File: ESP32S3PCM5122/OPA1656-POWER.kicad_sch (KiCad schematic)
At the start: 29 parts, among them IC6 TPS65133, U1 TPS7A39, U3 OPA1656

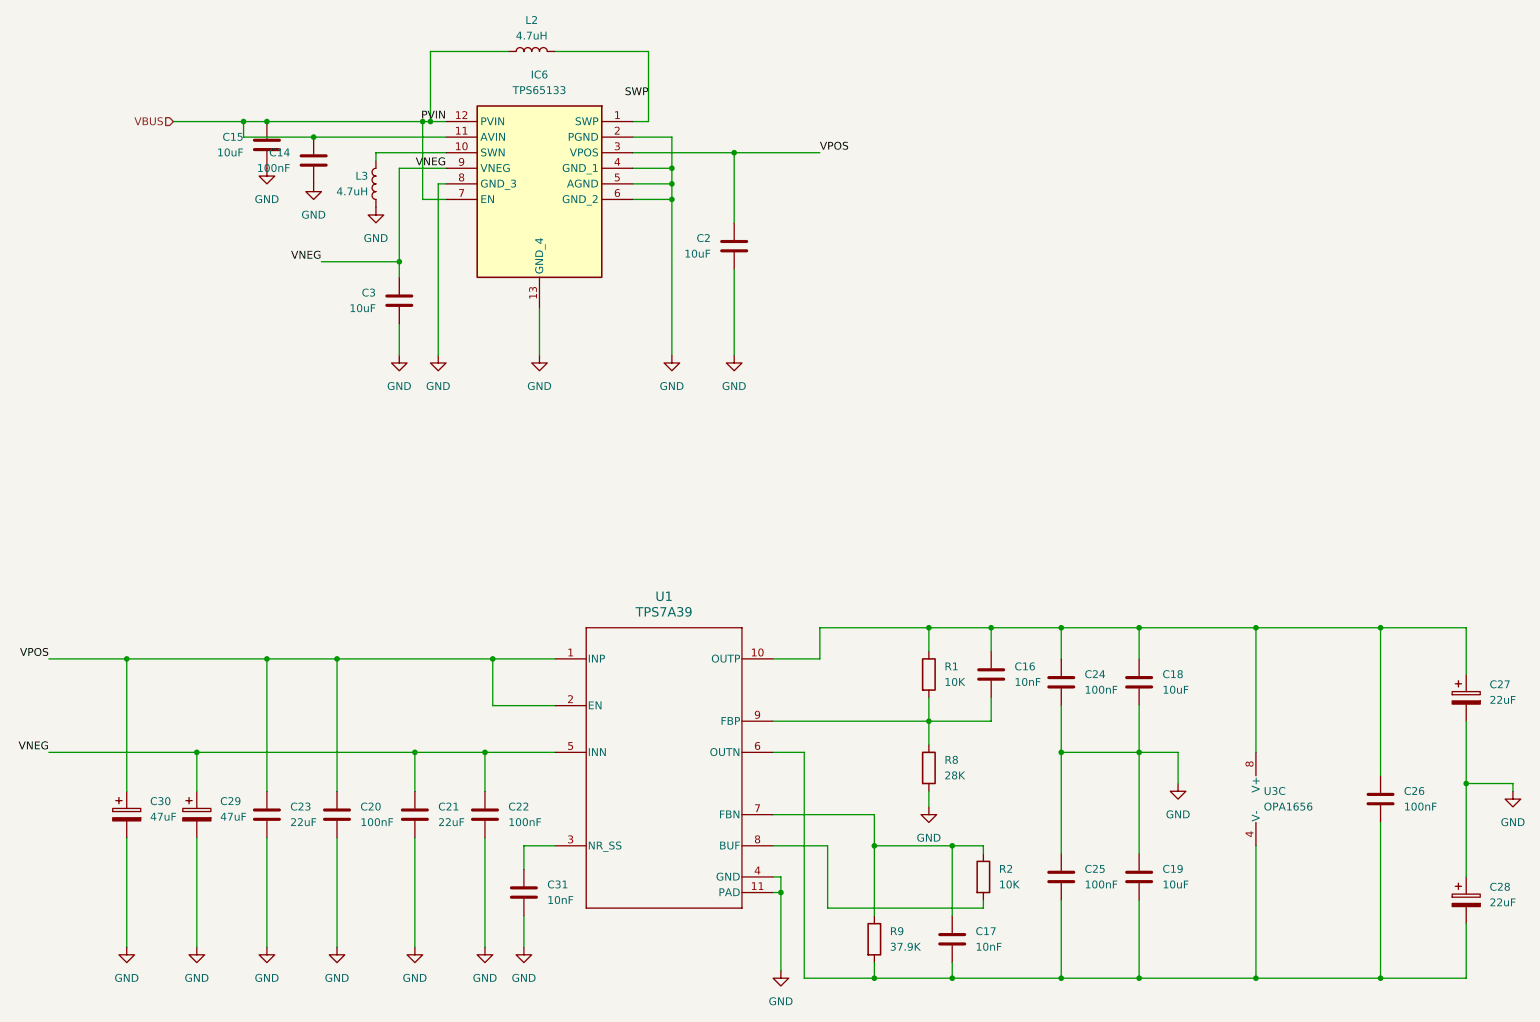
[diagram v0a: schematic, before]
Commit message: more work
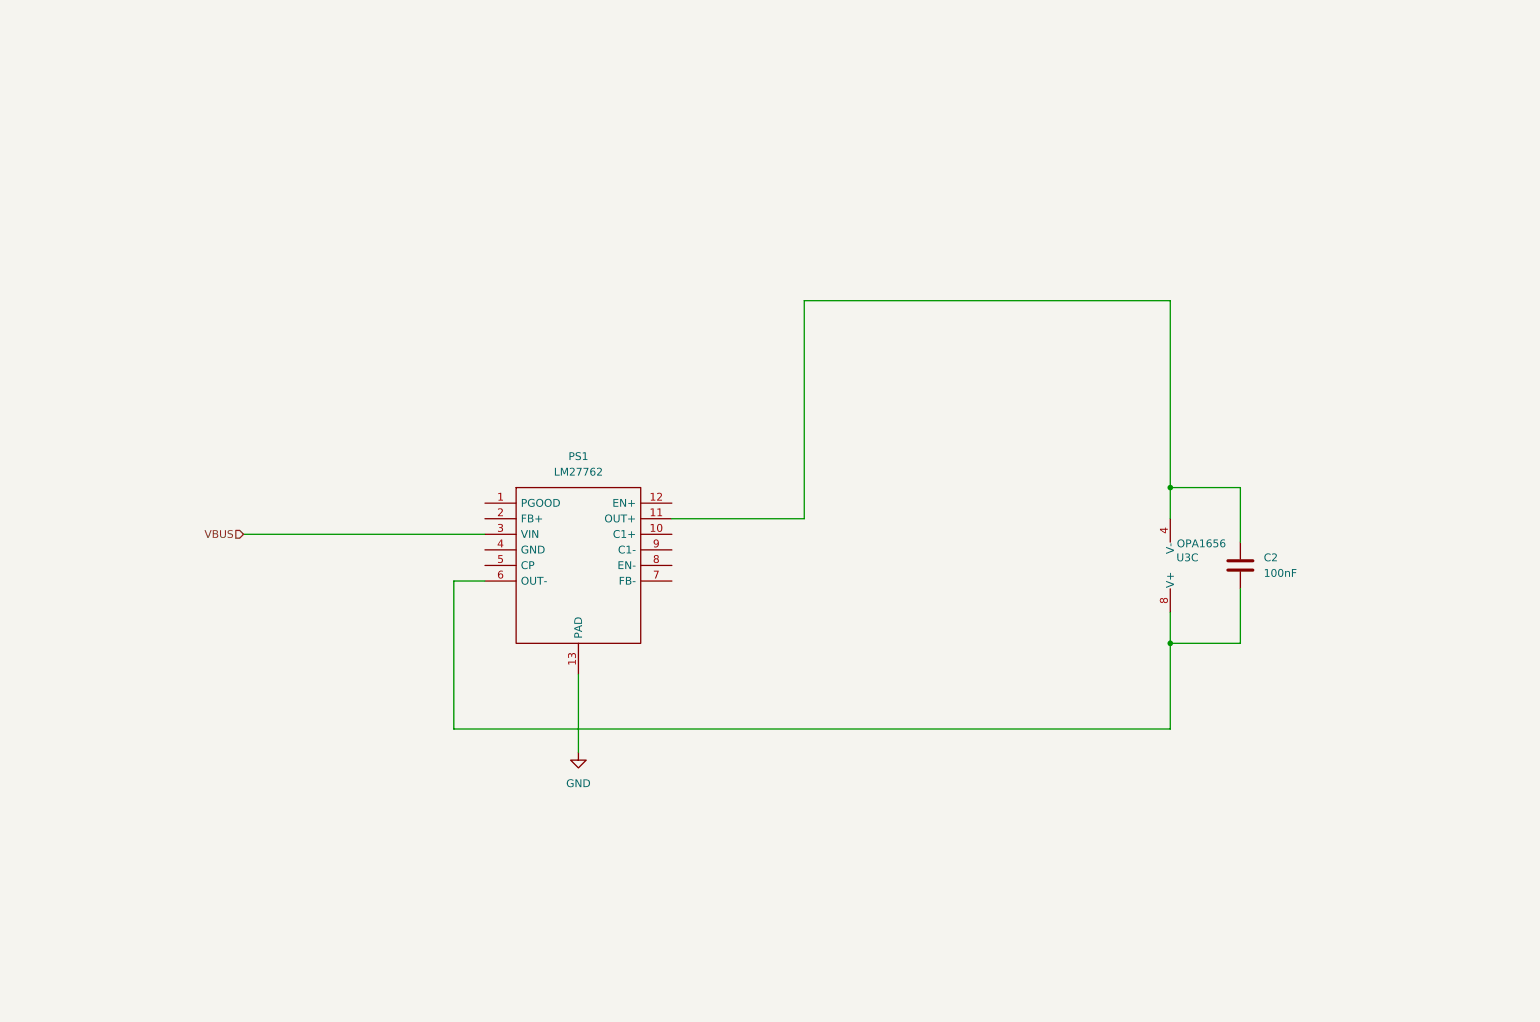
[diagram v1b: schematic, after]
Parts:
- removed C14, C20, C22, C24, C25, C26: 100nF, Capacitor_SMD:C_1206_3216Metric_Pad1.33x1.80mm_HandSolder, symbol Device:C
- removed C15, C18, C19, C3: 10uF, Capacitor_SMD:C_0805_2012Metric_Pad1.18x1.45mm_HandSolder, symbol Device:C
- removed C16, C17, C31: 10nF, Capacitor_SMD:C_0805_2012Metric_Pad1.18x1.45mm_HandSolder, symbol Device:C
- removed C21, C23: 22uF, Capacitor_SMD:C_1206_3216Metric_Pad1.33x1.80mm_HandSolder, symbol Device:C
- removed C27, C28: 22uF, Capacitor_THT:CP_Radial_D5.0mm_P2.50mm, symbol Device:C_Polarized
- removed C29, C30: 47uF, Capacitor_THT:CP_Radial_D5.0mm_P2.50mm, symbol Device:C_Polarized
- removed IC6: TPS65133, Custom:SON45P300X300X80-13N-D, symbol Custom:TPS65133DPDR
- removed L2, L3: 4.7uH, Inductor_SMD:L_1008_2520Metric_Pad1.43x2.20mm_HandSolder, symbol Device:L
- removed R1, R2: 10K, Resistor_SMD:R_0805_2012Metric_Pad1.20x1.40mm_HandSolder, symbol Device:R
- removed R8: 28K, Resistor_SMD:R_0805_2012Metric_Pad1.20x1.40mm_HandSolder, symbol Device:R
- removed R9: 37.9K, Resistor_SMD:R_0805_2012Metric_Pad1.20x1.40mm_HandSolder, symbol Device:R
- removed U1: TPS7A39, Custom:TPS7A3901DSCR, symbol Custom:TPS7A3901DSCR
- added PS1: LM27762, Custom:LM27762DSSR, symbol Custom:LM27762DSSR
- C2: value 10uF -> 100nF; footprint Capacitor_SMD:C_0805_2012Metric_Pad1.18x1.45mm_HandSolder -> Capacitor_SMD:C_1206_3216Metric_Pad1.33x1.80mm_HandSolder
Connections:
- net VPOS is gone; now on an unnamed net: C2.1
- net GND: now also PS1.13 (PAD); no longer C2.2
- net VBUS: now also PS1.3 (VIN)
- net at U3.8 (V+): now also C2.2, PS1.6 (OUT-)
- net at U3.4 (V-): now also PS1.11 (OUT+)
